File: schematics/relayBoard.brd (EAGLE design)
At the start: 79.7 x 69.8 mm, 20 parts, among them K1 AQG12105, K2 AQG12105

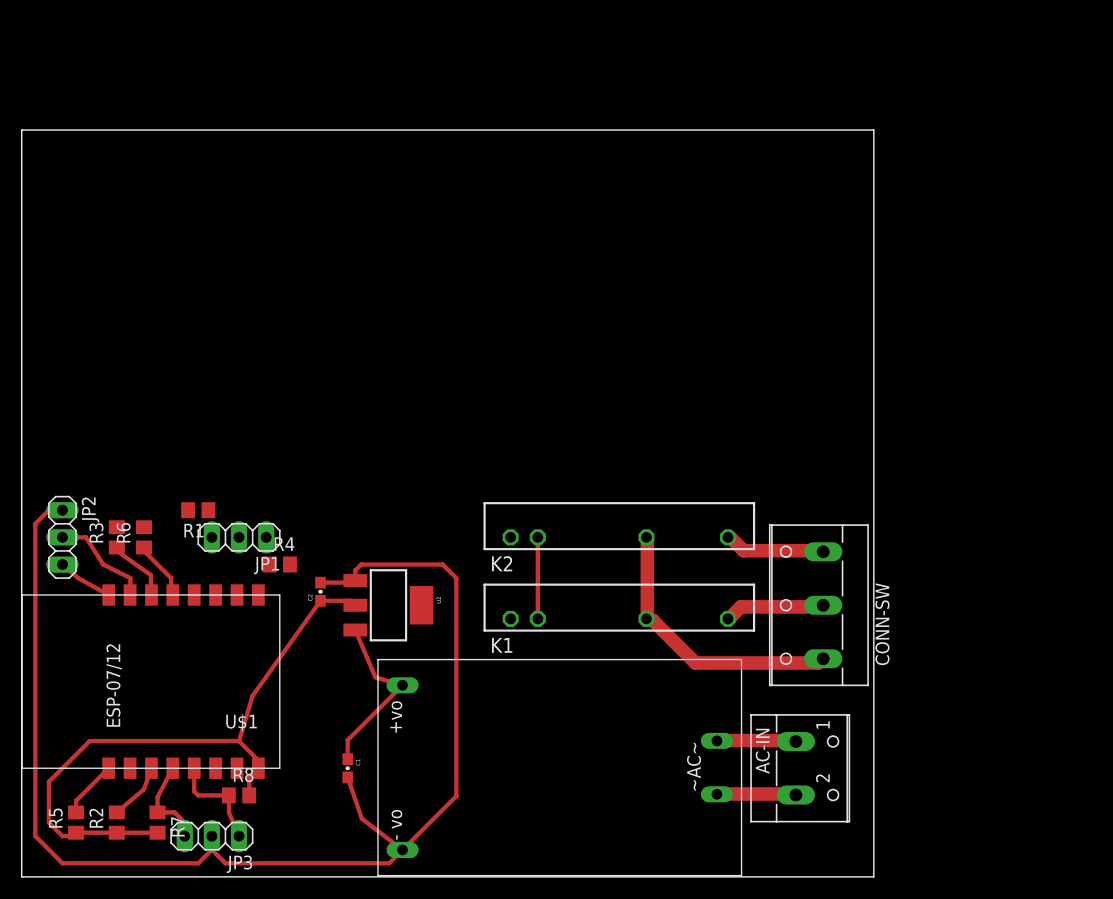
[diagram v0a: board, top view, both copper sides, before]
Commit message: code and schematic modifications
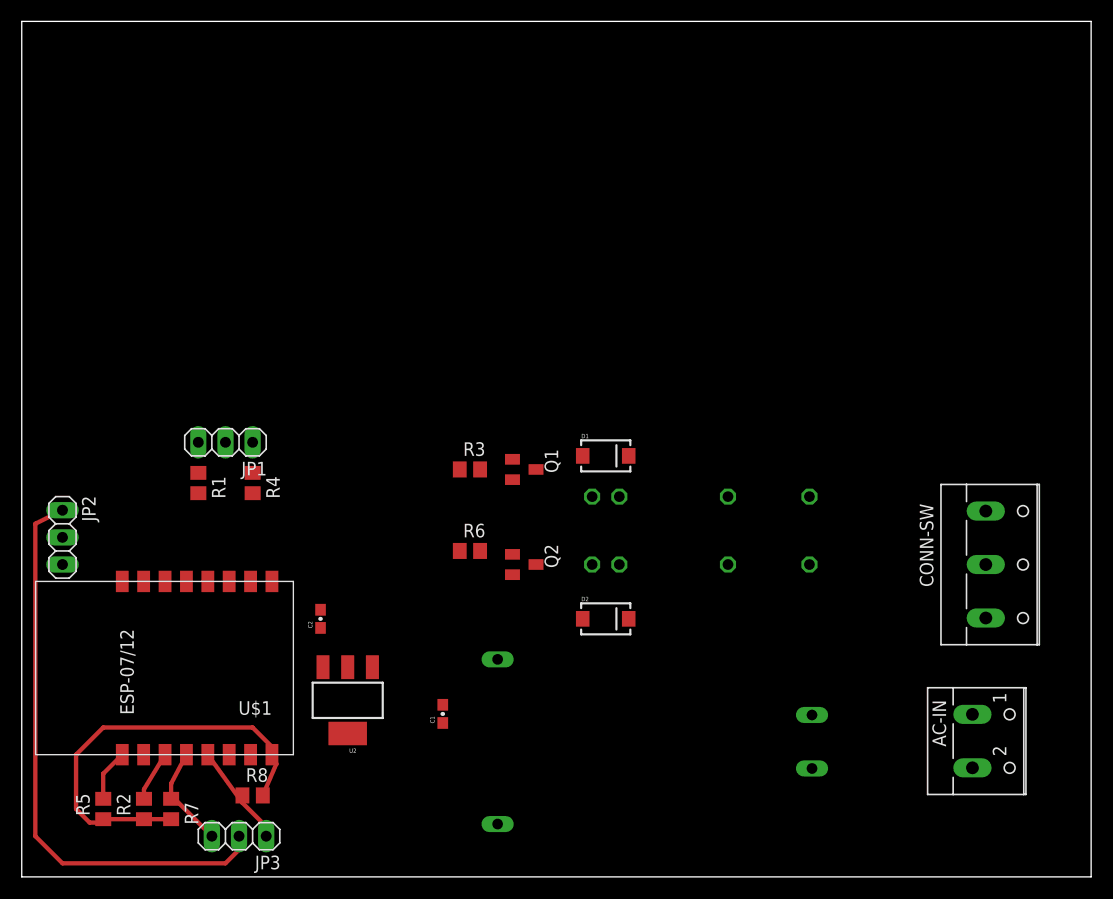
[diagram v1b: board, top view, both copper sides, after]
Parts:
- added D1, D2: (no value), SparkFun-DiscreteSemi:SMA-DIODE
- added Q1, Q2: (no value), semicon-smd-ipc:SOT23
- moved R3 33.6 mm to (41.9, 38.1), turned to 0 degrees
- moved R6 30.5 mm to (41.9, 30.5), turned to 0 degrees
- moved U$4 19.9 mm to (76.2, 2.54), flipped to the bottom, turned to 0 degrees
- moved CONN-SW 18.2 mm to (91.4, 29.2), turned to 270 degrees
- moved AC-IN 16.7 mm to (90.2, 12.7)
- moved K1 13.7 mm to (63.5, 35.6), flipped to the bottom, turned to 180 degrees
- moved C1 10.2 mm to (39.4, 15.2), turned to 90 degrees
- moved U2 9.67 mm to (30.5, 16.5), turned to 180 degrees
- moved JP1 8.98 mm to (19.1, 40.6)
- moved K2 8.03 mm to (63.5, 29.2), flipped to the bottom, turned to 180 degrees
- moved R4 8.03 mm to (21.6, 36.8), turned to 270 degrees
- moved R5 2.84 mm to (7.62, 6.35)
- moved R2 2.84 mm to (11.4, 6.35)
- moved C2 2.54 mm to (27.9, 24.1)
- moved JP3 2.54 mm to (20.3, 3.81)
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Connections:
- new net N$10: D1.A, K1.-, Q1.3
- new net N$12: Q1.1, R3.2
- new net N$7: D2.A, K2.-, Q2.3
- new net N$8: Q2.1, R6.2
- net 3V3: now also D1.C, D2.C; no longer R3.2, R6.2
- net GND: now also Q1.2, Q2.2
- net GPIO4: no longer K1.-
- net GPIO5: no longer K2.-
- net N$2: now also U$4.AC1; no longer U$4.AC2
- net N$5: now also U$4.AC2; no longer U$4.AC1
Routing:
- net GND: track 121.4 -> 53.9 mm
- net 3V3: track 66.6 -> 39.6 mm
- net AC-SW-L: track 26.1 -> 0.00 mm
- net 5V: track 16.5 -> 0.00 mm
- net RXD: track 9.64 -> 0.00 mm
- net LOAD2: track 9.45 -> 0.00 mm
- net LOAD1: track 9.41 -> 0.00 mm
- net N$5: track 7.41 -> 0.00 mm
- net N$2: track 7.41 -> 0.00 mm
- net GPIO4: track 6.09 -> 0.00 mm
- net GPIO5: track 5.56 -> 0.00 mm
- net TXD: track 5.20 -> 0.00 mm
- net GPIO16: track 8.69 -> 9.87 mm
- net CH_PD: track 5.42 -> 4.68 mm
- net GPIO14: track 9.56 -> 10.3 mm
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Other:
- board size 79.7 x 69.8 mm -> 100 x 80 mm
